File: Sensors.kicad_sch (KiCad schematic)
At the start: 18 parts, among them U12 ADXL375BCCZ-RL7, U2 MMC5983MA, U3 BMI088, U4 TMP275AIDGKR VSSOP8, U6 MS5607-02BA

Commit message: Chore: push new design
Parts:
- C30, C33, C36, C40, C42, C44, C48, C53, C58: footprint PCM_JLCPCB:C_0402 -> PCM_JLCPCB:C_0603
- R6: footprint PCM_JLCPCB:R_0402 -> PCM_JLCPCB:R_0603

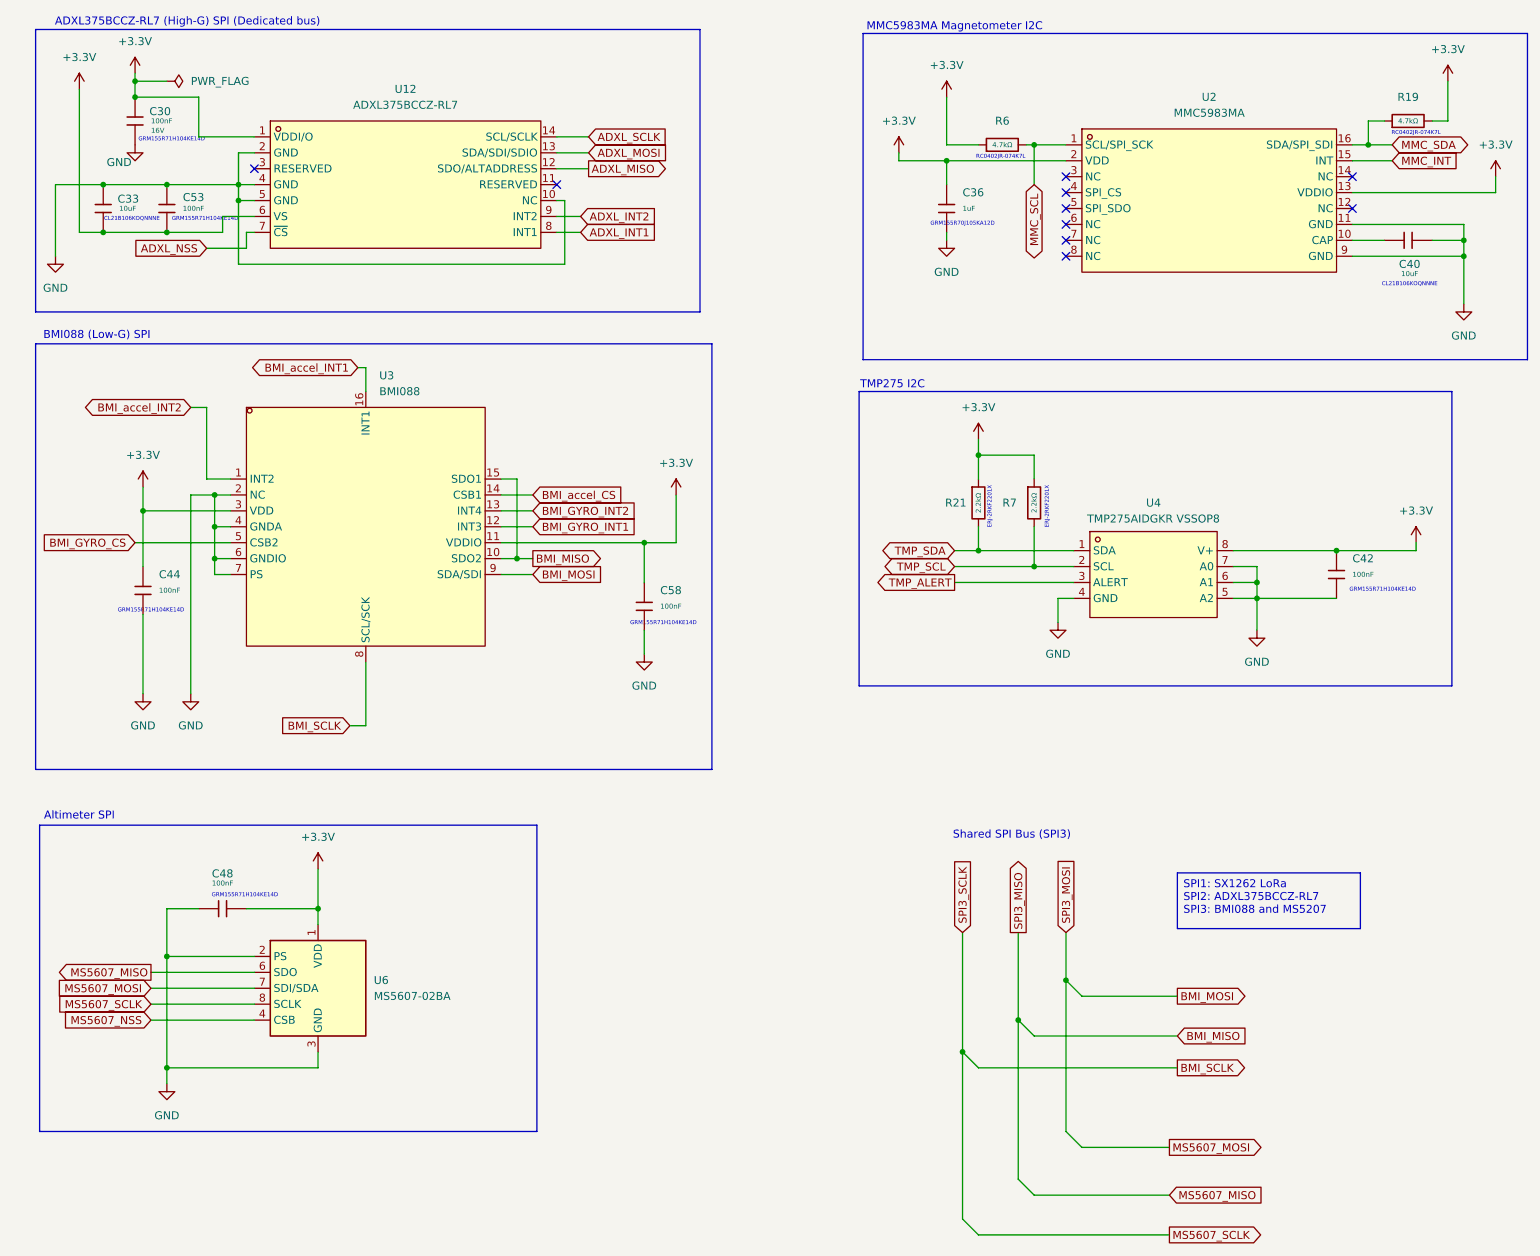
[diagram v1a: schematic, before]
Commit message: Special version
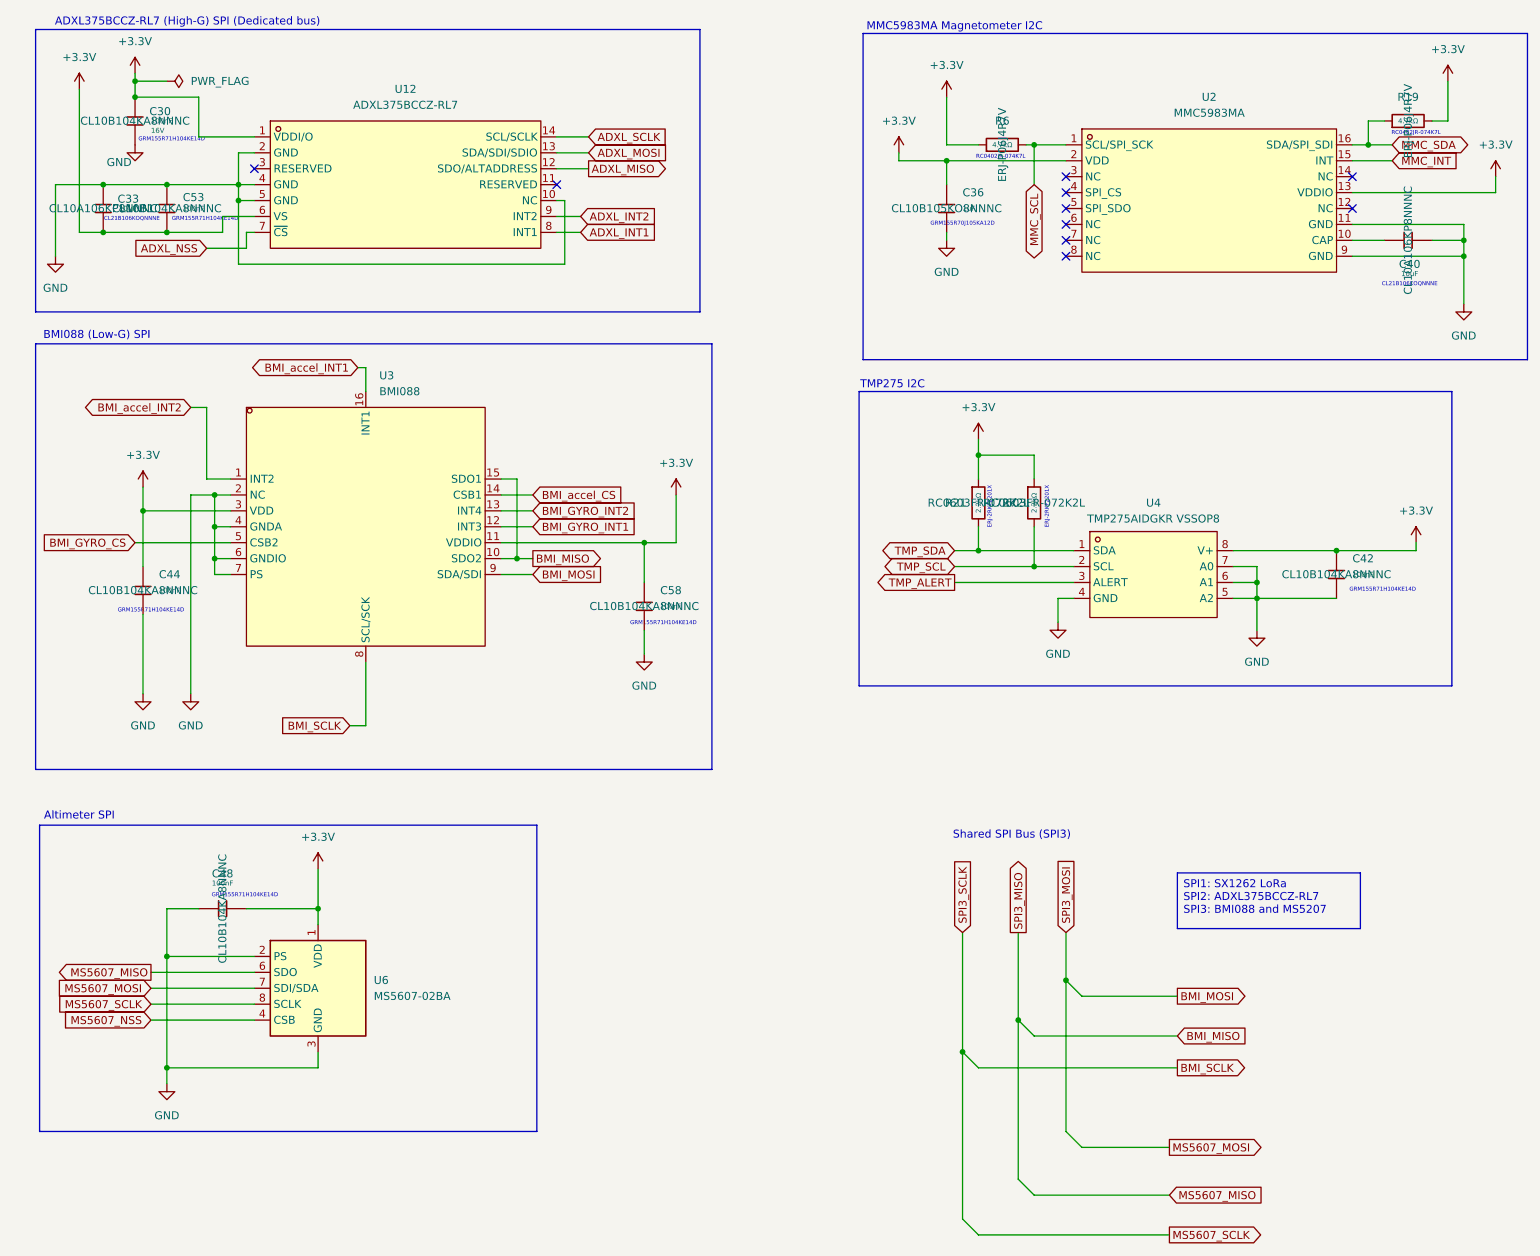
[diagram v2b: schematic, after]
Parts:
- C30, C42, C44, C48, C53, C58: Digikey Parts (none) -> CL10B104KA8NNNC
- C33, C40: Digikey Parts (none) -> CL10A106KP8NNNC
- C36: Digikey Parts (none) -> CL10B105KO8NNNC
- R19, R6: Digikey Parts (none) -> ERJ-P06J4R7V
- R21, R7: Digikey Parts (none) -> RC0603FR-072K2L
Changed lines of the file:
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@@
 			)
 		)
+		(property "Digikey Parts" "CL10B104KA8NNNC"
+			(at 36.83 45.72 0)
+			(effects
+				(font
+					(size 1.27 1.27)
+				)
+			)
+		)
 		(pin "2"
 		)
@@
 			)
 		)
+		(property "Digikey Parts" "CL10B104KA8NNNC"
+			(at 31.75 31.75 0)
+			(effects
+				(font
+					(size 1.27 1.27)
+				)
+			)
+		)
 		(pin "2"
 		)
@@
 			)
 		)
+		(property "Digikey Parts" "RC0603FR-072K2L"
+			(at 166.37 92.71 0)
+			(effects
+				(font
+					(size 1.27 1.27)
+				)
+			)
+		)
 		(pin "1"
 		)
@@
 			)
 		)
+		(property "Digikey Parts" "CL10B104KA8NNNC"
+			(at 45.72 157.48 0)
+			(effects
+				(font
+					(size 1.27 1.27)
+				)
+			)
+		)
 		(pin "1"
 		)
@@
 			)
 		)
+		(property "Digikey Parts" ""
+			(at 194.31 104.14 0)
+			(effects
+				(font
+					(size 1.27 1.27)
+				)
+			)
+		)
 		(pin "2"
 		)
@@
 			)
 		)
+		(property "Digikey Parts" "CL10B105KO8NNNC"
+			(at 161.29 45.72 0)
+			(effects
+				(font
+					(size 1.27 1.27)
+				)
+			)
+		)
 		(pin "2"
 		)
@@
 			)
 		)
+		(property "Digikey Parts" "CL10A106KP8NNNC"
+			(at 234.95 50.8 0)
+			(effects
+				(font
+					(size 1.27 1.27)
+				)
+			)
+		)
 		(pin "1"
 		)
@@
 			)
 		)
+		(property "Digikey Parts" "CL10B104KA8NNNC"
+			(at 113.03 109.22 0)
+			(effects
+				(font
+					(size 1.27 1.27)
+				)
+			)
+		)
 		(pin "2"
 		)
@@
 			)
 		)
+		(property "Digikey Parts" "RC0603FR-072K2L"
+			(at 175.26 92.71 0)
+			(effects
+				(font
+					(size 1.27 1.27)
+				)
+			)
+		)
 		(pin "1"
 		)
@@
 			)
 		)
+		(property "Digikey Parts" "ERJ-P06J4R7V"
+			(at 234.95 31.75 0)
+			(effects
+				(font
+					(size 1.27 1.27)
+				)
+			)
+		)
 		(pin "2"
 		)
@@
 			)
 		)
+		(property "Digikey Parts" ""
+			(at 203.2 44.45 0)
+			(effects
+				(font
+					(size 1.27 1.27)
+				)
+			)
+		)
 		(pin "2"
 		)
@@
 			)
 		)
+		(property "Digikey Parts" "ERJ-P06J4R7V"
+			(at 170.18 35.56 0)
+			(effects
+				(font
+					(size 1.27 1.27)
+				)
+			)
+		)
 		(pin "2"
 		)
@@
 			)
 		)
+		(property "Digikey Parts" ""
+			(at 60.96 170.18 0)
+			(effects
+				(font
+					(size 1.27 1.27)
+				)
+			)
+		)
 		(pin "7"
 		)
@@
 			)
 		)
+		(property "Digikey Parts" "CL10B104KA8NNNC"
+			(at 223.52 104.14 0)
+			(effects
+				(font
+					(size 1.27 1.27)
+				)
+			)
+		)
 		(pin "2"
 		)
@@
 			)
 		)
+		(property "Digikey Parts" ""
+			(at 68.58 96.52 0)
+			(effects
+				(font
+					(size 1.27 1.27)
+				)
+			)
+		)
 		(pin "4"
 		)
@@
 			)
 		)
+		(property "Digikey Parts" "CL10A106KP8NNNC"
+			(at 26.67 45.72 0)
+			(effects
+				(font
+					(size 1.27 1.27)
+				)
+			)
+		)
 		(pin "1"
 		)
@@
 			)
 		)
+		(property "Digikey Parts" ""
+			(at 74.93 41.91 0)
+			(effects
+				(font
+					(size 1.27 1.27)
+				)
+			)
+		)
 		(pin "2"
 		)
@@
 			(at 33.02 106.68 0)
 			(effects
+				(font
+					(size 1.27 1.27)
+				)
+			)
+		)
+		(property "Digikey Parts" "CL10B104KA8NNNC"
+			(at 33.02 106.68 0)
+			(effects
